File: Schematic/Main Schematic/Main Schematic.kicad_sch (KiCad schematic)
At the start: 5 parts, among them J2 Conn_01x24_Socket, J2 USB_B_Micro, J3 Conn_01x24_Socket, SW2 SW_Push

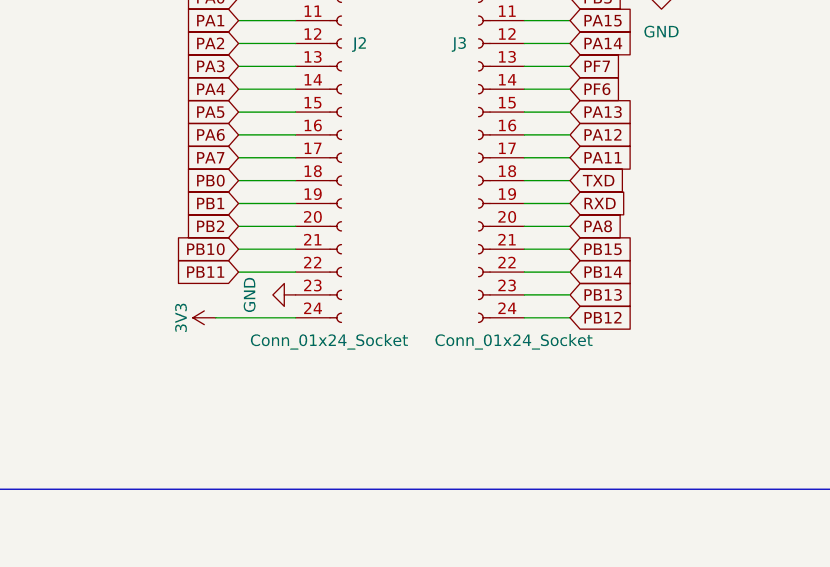
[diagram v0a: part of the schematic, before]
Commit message: 'Updated'
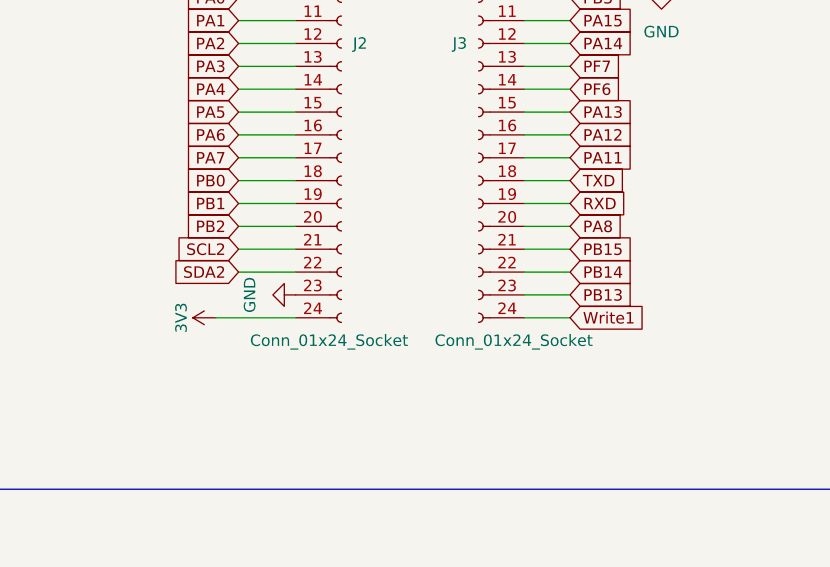
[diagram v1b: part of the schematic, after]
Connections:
- net PB10 renamed SCL2
- net PB11 renamed SDA2
- net PB12 renamed Write1
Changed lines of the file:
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@@
     )
   )
-  (global_label "PB12" (shape input) (at 255.27 88.9 0) (fields_autoplaced)
+  (global_label "Write1" (shape input) (at 255.27 88.9 0) (fields_autoplaced)
     (effects (font (size 1.27 1.27)) (justify left))
-    (property "Intersheetrefs" "${INTERSHEET_REFS}" (at 20.32 -64.77 0)
-      (effects (font (size 1.27 1.27)) hide)
+    (property "Intersheetrefs" "${INTERSHEET_REFS}" (at 264.042 88.9 0)
+      (effects (font (size 1.27 1.27)) (justify left) hide)
     )
   )
@@
     )
   )
-  (global_label "PB11" (shape input) (at 218.44 83.82 180) (fields_autoplaced)
+  (global_label "SDA2" (shape input) (at 218.44 83.82 180) (fields_autoplaced)
     (effects (font (size 1.27 1.27)) (justify right))
-    (property "Intersheetrefs" "${INTERSHEET_REFS}" (at 20.32 -64.77 0)
-      (effects (font (size 1.27 1.27)) hide)
+    (property "Intersheetrefs" "${INTERSHEET_REFS}" (at 210.7566 83.82 0)
+      (effects (font (size 1.27 1.27)) (justify right) hide)
     )
   )
@@
     )
   )
-  (global_label "PB10" (shape input) (at 218.44 81.28 180) (fields_autoplaced)
+  (global_label "SCL2" (shape input) (at 218.44 81.28 180) (fields_autoplaced)
     (effects (font (size 1.27 1.27)) (justify right))
-    (property "Intersheetrefs" "${INTERSHEET_REFS}" (at 20.32 -64.77 0)
-      (effects (font (size 1.27 1.27)) hide)
+    (property "Intersheetrefs" "${INTERSHEET_REFS}" (at 210.8171 81.28 0)
+      (effects (font (size 1.27 1.27)) (justify right) hide)
     )
   )
